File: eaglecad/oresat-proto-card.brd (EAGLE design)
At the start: 99.8 x 94.7 mm, 263 parts, among them J6 J-SAMTEC-TFM-120-X1-XXX-D-RA, Q10 DMP2240UDM, Q11 MOSFET-PCH-SOT23-6, Q12 MOSFET-PCH-SOT23-6, Q13 PMV45EN, Q14 PMV45EN, Q15 DMP2240UDM, Q16 MOSFET-PCH-SOT23-6, Q17 MOSFET-PCH-SOT23-6, Q18 PMV45EN, Q19 PMV45EN, Q20 DMP2240UDM, Q21 MOSFET-PCH-SOT23-6, Q22 MOSFET-PCH-SOT23-6, Q23 PMV45EN, Q24 PMV45EN, Q25 DMP2240UDM, Q6 MOSFET-PCH-SOT23-6, Q7 MOSFET-PCH-SOT23-6, Q8 PMV45EN, Q9 PMV45EN, U10 MAX7310ATE, U11 MAX4211CETE, U12 MCP1703A, U13 MAX7310ATE, U14 MAX4211CETE, U15 MCP1703A, U3 MAX7310ATE, U4 MAX4211CETE, U6 MCP1703A, U7 MAX7310ATE, U8 MAX4211CETE, U9 MCP1703A

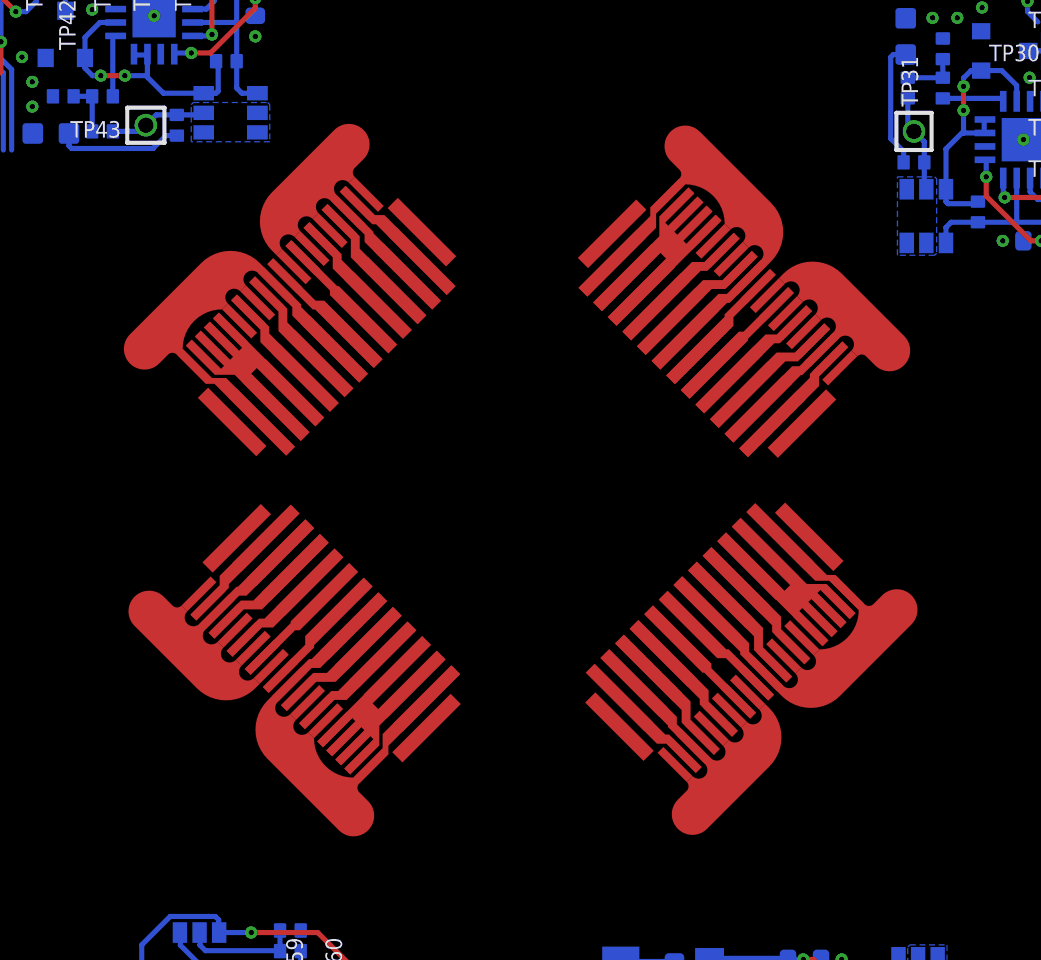
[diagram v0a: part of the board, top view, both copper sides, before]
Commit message: connector update
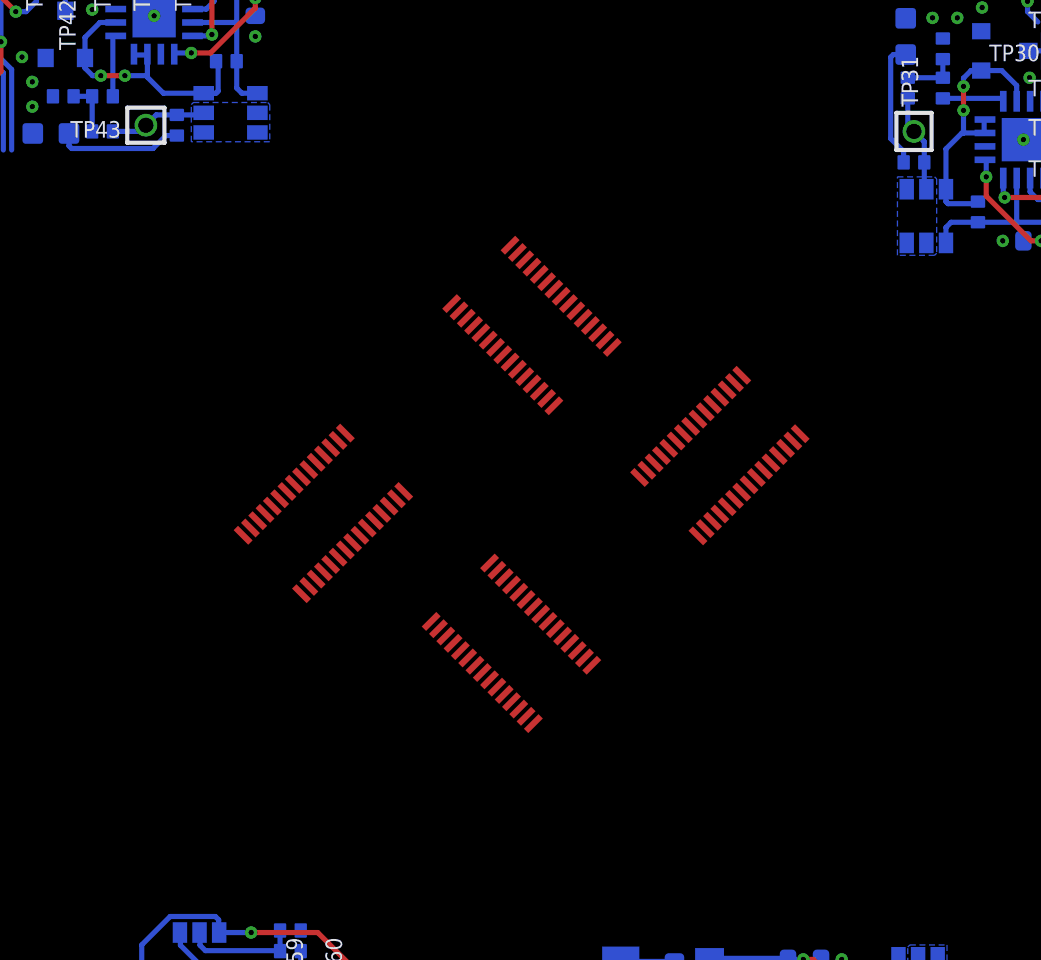
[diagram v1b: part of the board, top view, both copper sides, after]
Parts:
- U$1, U$3, U$4, U$5: value CARD-FLEX_CONNCARD-FLEX_CONN -> MEZZANINE_1; device oresat-ACS_driver_board:10-8_STAGGERED-PAD_CARD_CONN -> oresat-ACS_driver_board:MEZZANINE_1
- moved U$4 10.9 mm to (40.3, 48.5), turned to 45 degrees
- moved U$5 10.6 mm to (49.4, 42.2), turned to 135 degrees
- moved U$3 10.4 mm to (59.5, 51.3), turned to 45 degrees
- moved U$1 10.4 mm to (50.4, 57.6), turned to 315 degrees
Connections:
- net BOOT_Q1: now also U$3.P$22, U$3.P$9; no longer U$3.BOOT1, U$3.BOOT2
- net BOOT_Q2: now also U$1.P$22, U$1.P$9; no longer U$1.BOOT1, U$1.BOOT2
- net BOOT_Q3: now also U$4.P$22, U$4.P$9; no longer U$4.BOOT1, U$4.BOOT2
- net BOOT_Q4: now also U$5.P$22, U$5.P$9; no longer U$5.BOOT1, U$5.BOOT2
- net CAN2_H: now also U$1.P$25, U$1.P$6, U$3.P$25, U$3.P$6, U$4.P$25, U$4.P$6, U$5.P$25, U$5.P$6; no longer U$1.CAN_H1, U$1.CAN_H2, U$3.CAN_H1, U$3.CAN_H2, U$4.CAN_H1, U$4.CAN_H2, U$5.CAN_H1, U$5.CAN_H2
- net CAN2_L: now also U$1.P$26, U$1.P$5, U$3.P$26, U$3.P$5, U$4.P$26, U$4.P$5, U$5.P$26, U$5.P$5; no longer U$1.CAN_L1, U$1.CAN_L2, U$3.CAN_L1, U$3.CAN_L2, U$4.CAN_L1, U$4.CAN_L2, U$5.CAN_L1, U$5.CAN_L2
- net GND: now also U$1.P$1, U$1.P$14, U$1.P$15, U$1.P$16, U$1.P$17, U$1.P$2, U$1.P$29, U$1.P$30, U$3.P$1, U$3.P$14, U$3.P$15, U$3.P$16, U$3.P$17, U$3.P$2, U$3.P$29, U$3.P$30, U$4.P$1, U$4.P$14, U$4.P$15, U$4.P$16, U$4.P$17, U$4.P$2, U$4.P$29, U$4.P$30, U$5.P$1, U$5.P$14, U$5.P$15, U$5.P$16, U$5.P$17, U$5.P$2, U$5.P$29, U$5.P$30; no longer U$1.GND1, U$1.GND10, U$1.GND11, U$1.GND12, U$1.GND13, U$1.GND14, U$1.GND2, U$1.GND3, U$1.GND4, U$1.GND5, U$1.GND6, U$1.GND7, U$1.GND8, U$1.GND9, U$3.GND1, U$3.GND10, U$3.GND11, U$3.GND12, U$3.GND13, U$3.GND14, U$3.GND2, U$3.GND3, U$3.GND4, U$3.GND5, U$3.GND6, U$3.GND7, U$3.GND8, U$3.GND9, U$4.GND1, U$4.GND10, U$4.GND11, U$4.GND12, U$4.GND13, U$4.GND14, U$4.GND2, U$4.GND3, U$4.GND4, U$4.GND5, U$4.GND6, U$4.GND7, U$4.GND8, U$4.GND9, U$5.GND1, U$5.GND10, U$5.GND11, U$5.GND12, U$5.GND13, U$5.GND14, U$5.GND2, U$5.GND3, U$5.GND4, U$5.GND5, U$5.GND6, U$5.GND7, U$5.GND8, U$5.GND9
- net MAG1_Q1: now also U$3.P$10, U$3.P$21; no longer U$3.MAG11, U$3.MAG12
- net MAG1_Q2: now also U$1.P$10, U$1.P$21; no longer U$1.MAG11, U$1.MAG12
- net MAG1_Q3: now also U$4.P$10, U$4.P$21; no longer U$4.MAG11, U$4.MAG12
- net MAG1_Q4: now also U$5.P$10, U$5.P$21; no longer U$5.MAG11, U$5.MAG12
- net MAG2_Q1: now also U$3.P$11, U$3.P$20; no longer U$3.MAG21, U$3.MAG22
- net MAG2_Q2: now also U$1.P$11, U$1.P$20; no longer U$1.MAG21, U$1.MAG22
- net MAG2_Q3: now also U$4.P$11, U$4.P$20; no longer U$4.MAG21, U$4.MAG22
- net MAG2_Q4: now also U$5.P$11, U$5.P$20; no longer U$5.MAG21, U$5.MAG22
- net SCL_Q1: now also U$3.P$24, U$3.P$7; no longer U$3.SCL1, U$3.SCL2
- net SCL_Q2: now also U$1.P$24, U$1.P$7; no longer U$1.SCL1, U$1.SCL2
- net SCL_Q3: now also U$4.P$24, U$4.P$7; no longer U$4.SCL1, U$4.SCL2
- net SCL_Q4: now also U$5.P$24, U$5.P$7; no longer U$5.SCL1, U$5.SCL2
- net SDA_Q1: now also U$3.P$23, U$3.P$8; no longer U$3.SDA1, U$3.SDA2
- net SDA_Q2: now also U$1.P$23, U$1.P$8; no longer U$1.SDA1, U$1.SDA2
- net SDA_Q3: now also U$4.P$23, U$4.P$8; no longer U$4.SDA1, U$4.SDA2
- net SDA_Q4: now also U$5.P$23, U$5.P$8; no longer U$5.SDA1, U$5.SDA2
- net VBUSP_Q1: now also U$3.P$12, U$3.P$13, U$3.P$18, U$3.P$19, U$3.P$27, U$3.P$28, U$3.P$3, U$3.P$4; no longer U$3.VCC1, U$3.VCC2, U$3.VCC3, U$3.VCC4, U$3.VCC5, U$3.VCC6
- net VBUSP_Q2: now also U$1.P$12, U$1.P$13, U$1.P$18, U$1.P$19, U$1.P$27, U$1.P$28, U$1.P$3, U$1.P$4; no longer U$1.VCC1, U$1.VCC2, U$1.VCC3, U$1.VCC4, U$1.VCC5, U$1.VCC6
- net VBUSP_Q3: now also U$4.P$12, U$4.P$13, U$4.P$18, U$4.P$19, U$4.P$27, U$4.P$28, U$4.P$3, U$4.P$4; no longer U$4.VCC1, U$4.VCC2, U$4.VCC3, U$4.VCC4, U$4.VCC5, U$4.VCC6
- net VBUSP_Q4: now also U$5.P$12, U$5.P$13, U$5.P$18, U$5.P$19, U$5.P$27, U$5.P$28, U$5.P$3, U$5.P$4; no longer U$5.VCC1, U$5.VCC2, U$5.VCC3, U$5.VCC4, U$5.VCC5, U$5.VCC6
